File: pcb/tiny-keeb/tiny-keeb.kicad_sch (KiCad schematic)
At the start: 124 parts, among them J2 Conn_01x20_Socket, SW1 SW_RCTRL, SW10 SW_A, SW11 SW_X, SW12 SW_LWIN, SW13 SW_2, SW14 SW_E, SW15 SW_S, SW16 SW_C, SW17 SW_LALT, SW18 SW_', SW19 SW_3, SW2 SW_ESC, SW20 SW_R, SW21 SW_D, SW22 SW_V, SW23 SW_Z, SW24 SW_/, SW25 SW_4, SW26 SW_T, SW27 SW_F, SW28 SW_B, SW29 SW_-, SW3 SW_TAB, SW30 SW_SPACE2, SW31 SW_5, SW32 SW_Y, SW33 SW_G, SW34 SW_N, SW35 SW_], SW37 SW_6, SW38 SW_U, SW39 SW_H, SW4 SW_CAPS, SW40 SW_M, SW41 SW_SPACE, SW43 SW_7, SW44 SW_I, SW45 SW_J, SW46 SW_,, SW49 SW_8, SW5 SW_LSHIFT, SW50 SW_O, SW51 SW_K, SW52 SW_., SW55 SW_9, SW56 SW_P, SW57 SW_L, SW58 SW_RSHIFT, SW59 SW_RALT, SW6 SW_LCTRL, SW61 SW_0, SW62 SW_[, SW63 SW_;, SW65 SW_RWIN, SW66 SW_FN, SW67 SW_=, SW7 SW_Q, SW72 SW_BACKSPACE, SW73 SW_\, SW74 SW_ENTER, SW8 SW_1, SW9 SW_W

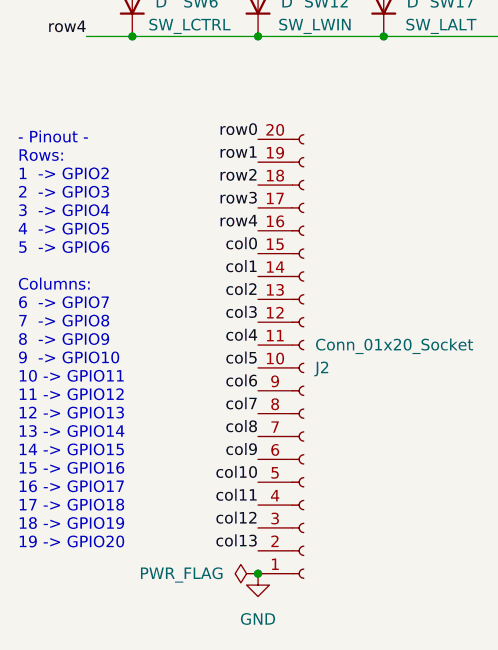
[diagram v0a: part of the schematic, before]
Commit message: minor fixes, first board built, add pictures later and release
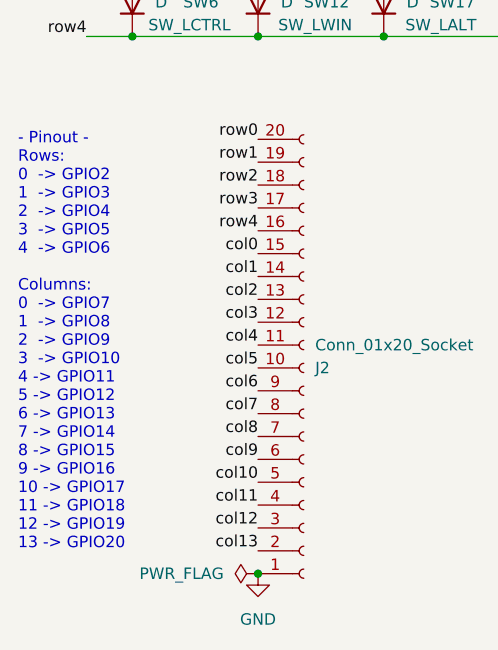
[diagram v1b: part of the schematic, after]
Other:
- note added: "- Pinout - Rows: 0 -> GPIO2 1 -> GPIO3 2 -> GPIO4 3 -> GPIO5 4 -> GPIO6 Columns: 0 -> GPIO7 1 -> GPIO8 2 -> GPIO9 3 -> GPIO10 4 -> GPIO11 5 -> GPIO12 6 -> GPIO13 7 -> GPIO14 8 -> GPIO15 9 -> GPIO16 10 -> GPIO17 11 -> GPIO18 12 -> GPIO19 13 -> GPIO20"
- note removed: "- Pinout - Rows: 1 -> GPIO2 2 -> GPIO3 3 -> GPIO4 4 -> GPIO5 5 -> GPIO6 Columns: 6 -> GPIO7 7 -> GPIO8 8 -> GPIO9 9 -> GPIO10 10 -> GPIO11 11 -> GPIO12 12 -> GPIO13 13 -> GPIO14 14 -> GPIO15 15 -> GPIO16 16 -> GPIO17 17 -> GPIO18 18 -> GPIO19 19 -> GPIO20"
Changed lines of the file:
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@@
     (stroke (width 0) (type default))
   )
-  (text "- Pinout - \nRows:\n1  -> GPIO2\n2  -> GPIO3\n3  -> GPIO4\n4  -> GPIO5\n5  -> GPIO6\n\nColumns:\n6  -> GPIO7\n7  -> GPIO8\n8  -> GPIO9\n9  -> GPIO10\n10 -> GPIO11\n11 -> GPIO12\n12 -> GPIO13\n13 -> GPIO14\n14 -> GPIO15\n15 -> GPIO16\n16 -> GPIO17\n17 -> GPIO18\n18 -> GPIO19\n19 -> GPIO20"
+  (text "- Pinout - \nRows:\n0  -> GPIO2\n1  -> GPIO3\n2  -> GPIO4\n3  -> GPIO5\n4  -> GPIO6\n\nColumns:\n0  -> GPIO7\n1  -> GPIO8\n2  -> GPIO9\n3  -> GPIO10\n4 -> GPIO11\n5 -> GPIO12\n6 -> GPIO13\n7 -> GPIO14\n8 -> GPIO15\n9 -> GPIO16\n10 -> GPIO17\n11 -> GPIO18\n12 -> GPIO19\n13 -> GPIO20"
     (at 21.59 158.75 0)
     (effects (font (size 1.27 1.27)) (justify left bottom))
